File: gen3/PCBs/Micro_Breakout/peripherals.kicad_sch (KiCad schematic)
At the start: 88 parts, among them J10 Conn_02x03_Odd_Even, J11 430450422, J12 PixHawk PM02, J14 Conn_01x02_Socket, J17 430450422, J18 430450422, J19 430450422, J2 430450422, J20 430450228, J21 430450228, J22 430450228, J23 430450228, J25 430450228, J26 430450821, J28 Conn_01x04_Socket, J3 Conn_01x03_Pin, J31 Conn_01x02_Socket, J4 430450422, J5 430451027, J8 Conn_02x22_Odd_Even, J9 J1B1211CCD

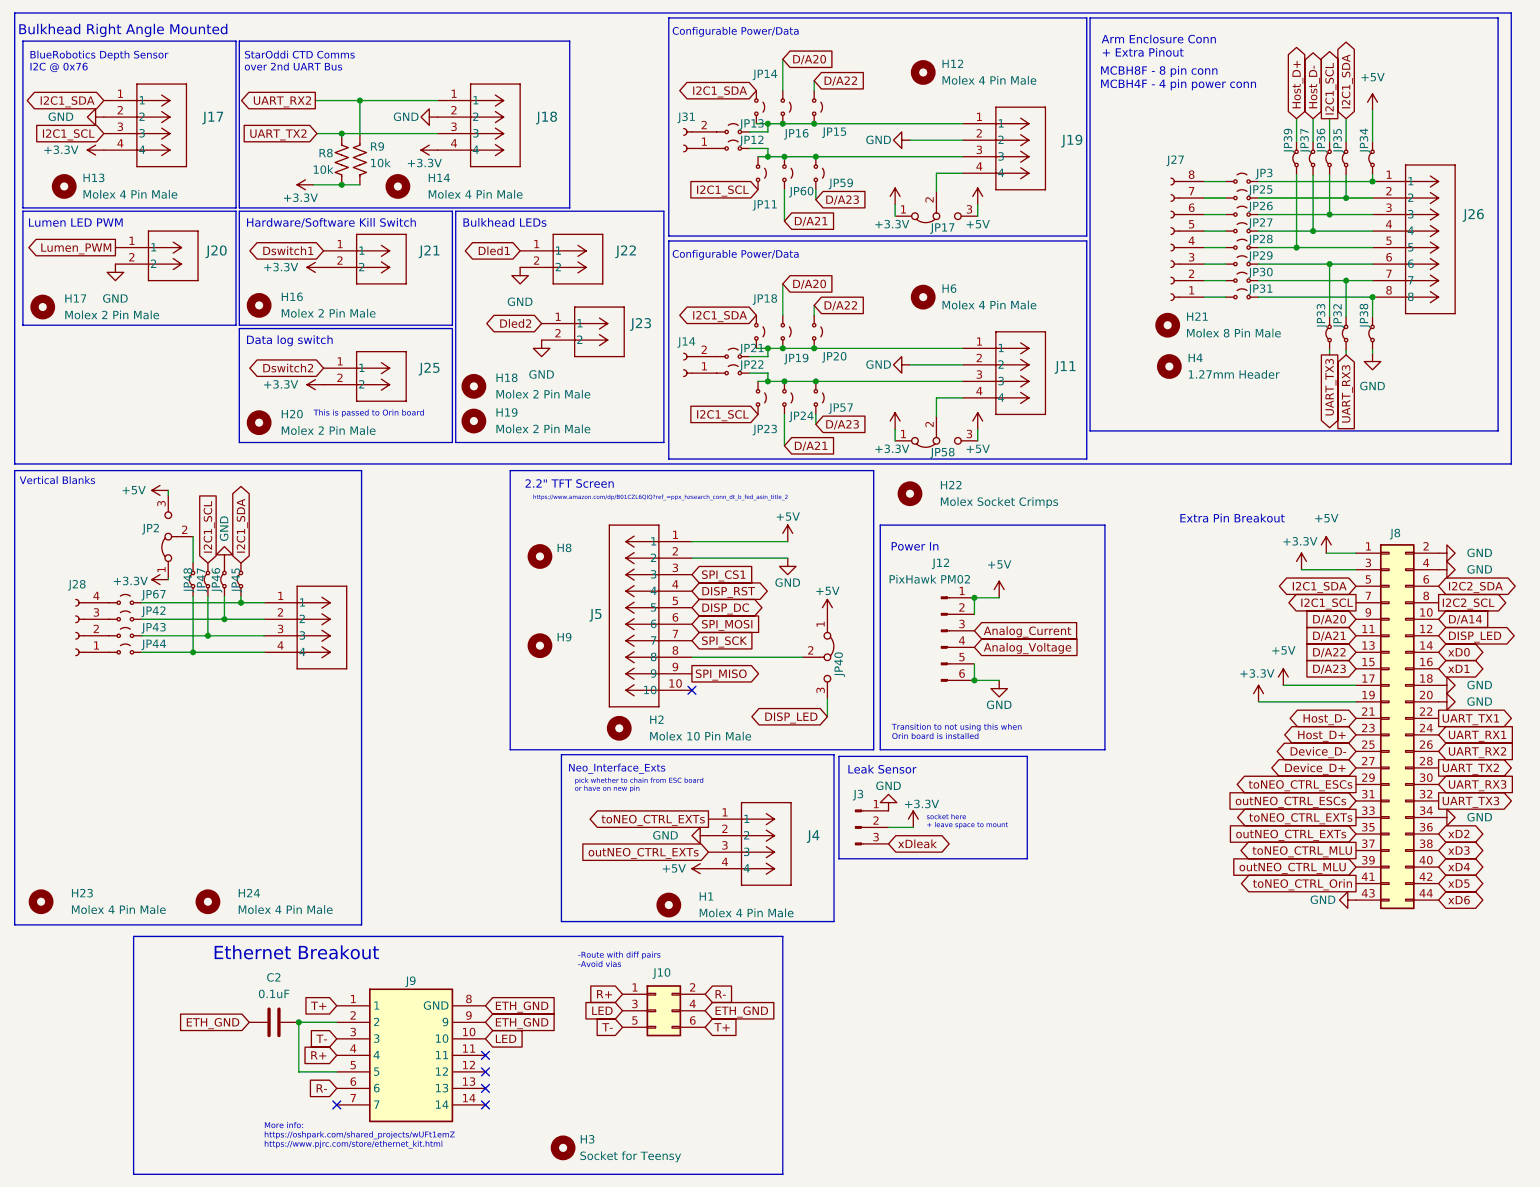
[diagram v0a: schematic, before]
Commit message: initial designs
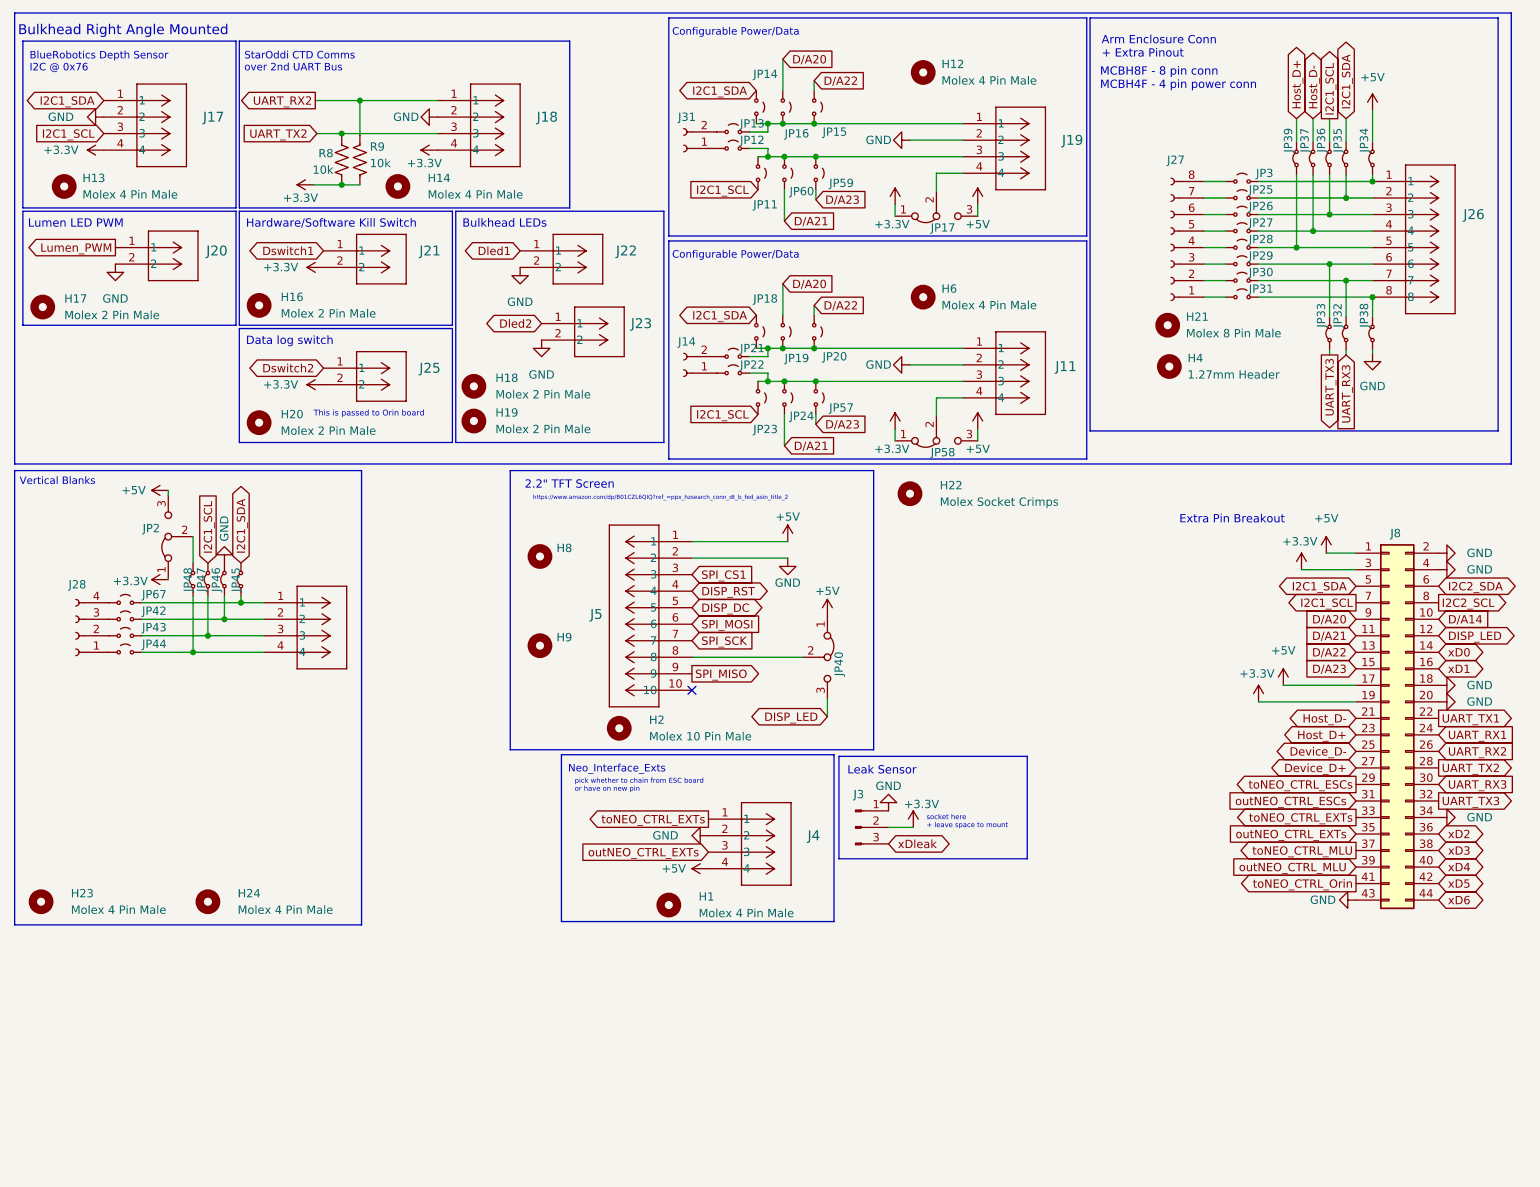
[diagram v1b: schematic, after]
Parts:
- removed C2: 0.1uF, ImportedV2:K104K15X7RF5TL2_VIS, symbol Device:C
- removed H3: Socket for Teensy, symbol Mechanical:MountingHole
- removed J10: Conn_02x03_Odd_Even, Connector_PinHeader_2.00mm:PinHeader_2x03_P2.00mm_Vertical, symbol Connector_Generic:Conn_02x03_Odd_Even
- removed J12: PixHawk PM02, Connector_PinSocket_2.54mm:PinSocket_1x06_P2.54mm_Vertical, symbol Connector:Conn_01x06_Pin
- removed J9: J1B1211CCD, ImportedV2:J1B1211CCD, symbol Imported:J1B1211CCD
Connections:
- no-connect marks 6 -> 1
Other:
- note removed: "-Route with diff pairs -Avoid vias"
- note removed: "Ethernet Breakout"
- note removed: "More info: https://oshpark.com/shared_projects/wUFt1emZ https://www.pjrc.com/store/ethernet_kit.html"
- note removed: "Power In"
- note removed: "Transition to not using this when Orin board is installed"
